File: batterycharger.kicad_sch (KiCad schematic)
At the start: 0 parts

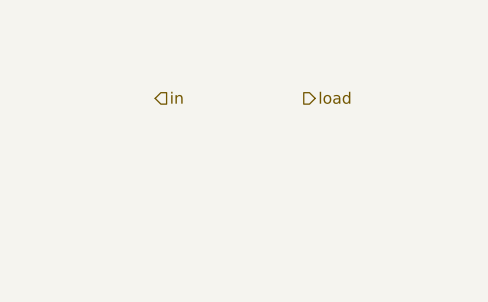
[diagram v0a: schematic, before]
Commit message: added
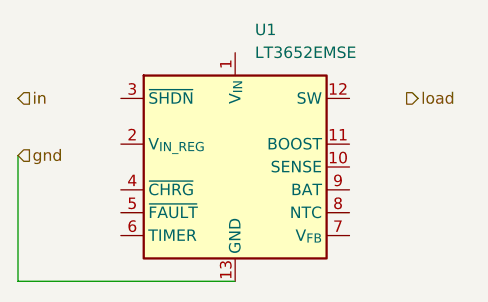
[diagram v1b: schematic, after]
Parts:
- added U1: LT3652EMSE, Package_SO:MSOP-12-1EP_3x4mm_P0.65mm_EP1.65x2.85mm, symbol Battery_Management:LT3652EMSE
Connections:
- new net gnd: U1.13 (GND)
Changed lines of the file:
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@@
 (kicad_sch (version 20230121) (generator eeschema)
   (paper "A4")
-  (hierarchical_label "in" (shape input) (at 78.74 87.63 0) (fields_autoplaced)
+  (wire (pts (xy 63.5 107.95) (xy 87.63 107.95))
+    (stroke (width 0) (type default))
+  )
+  (wire (pts (xy 63.5 93.98) (xy 63.5 107.95))
+    (stroke (width 0) (type default))
+  )
+  (hierarchical_label "in" (shape input) (at 63.5 87.63 0) (fields_autoplaced)
     (effects (font (size 1.27 1.27)) (justify left))
   )
-  (hierarchical_label "load" (shape output) (at 95.25 87.63 0) (fields_autoplaced)
+  (hierarchical_label "gnd" (shape input) (at 63.5 93.98 0) (fields_autoplaced)
     (effects (font (size 1.27 1.27)) (justify left))
   )
+  (hierarchical_label "load" (shape output) (at 106.68 87.63 0) (fields_autoplaced)
+    (effects (font (size 1.27 1.27)) (justify left))
+  )
+  (symbol (lib_id "Battery_Management:LT3652EMSE") (at 87.63 95.25 0) (unit 1)
+    (in_bom yes) (on_board yes) (dnp no) (fields_autoplaced)
+    (property "Reference" "U1" (at 89.8241 80.01 0)
+      (effects (font (size 1.27 1.27)) (justify left))
+    )
+    (property "Value" "LT3652EMSE" (at 89.8241 82.55 0)
+      (effects (font (size 1.27 1.27)) (justify left))
+    )
+    (property "Footprint" "Package_SO:MSOP-12-1EP_3x4mm_P0.65mm_EP1.65x2.85mm" (at 87.63 110.49 0)
+      (effects (font (size 1.27 1.27)) hide)
+    )
+    (property "Datasheet" "https://www.analog.com/media/en/technical-documentation/data-sheets/3652fe.pdf" (at 102.87 115.57 0)
+      (effects (font (size 1.27 1.27)) hide)
+    )
+    (pin "1")
+    (pin "10")
+    (pin "11")
+    (pin "12")
+    (pin "13")
+    (pin "2")
+    (pin "3")
+    (pin "4")
+    (pin "5")
+    (pin "6")
+    (pin "7")
+    (pin "8")
+    (pin "9")
+    (instances
+      (project "eps"
+        (path "/d1becec8-2a81-45a7-bfc6-f9ad93456edc/a41c2f06-c716-4d4c-abbd-50372b3cec58"
+          (reference "U1") (unit 1)
+        )
+        (path "/d1becec8-2a81-45a7-bfc6-f9ad93456edc/98043307-5f00-404c-bb35-46ff24bbd3b8"
+          (reference "U2") (unit 1)
+        )
+      )
+    )
+  )
 )

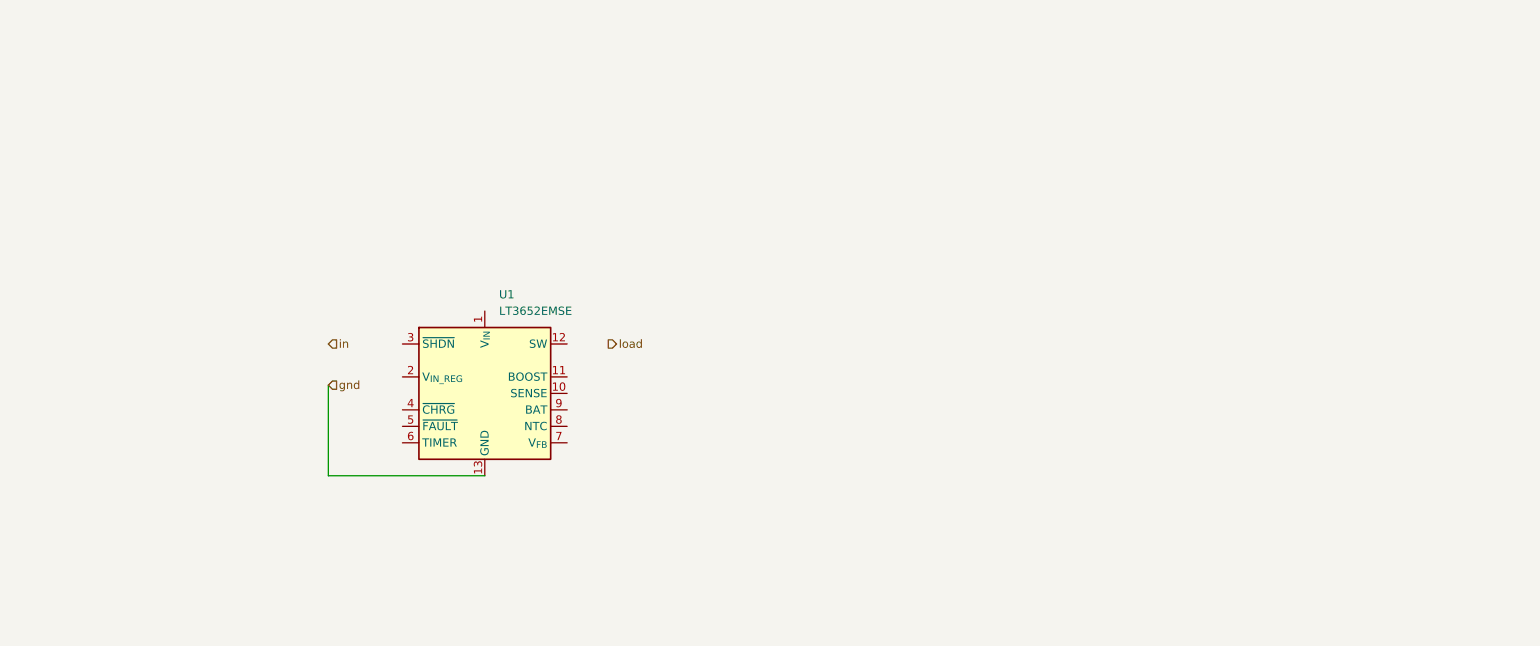
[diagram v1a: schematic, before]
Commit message: v0.1Hydrogen
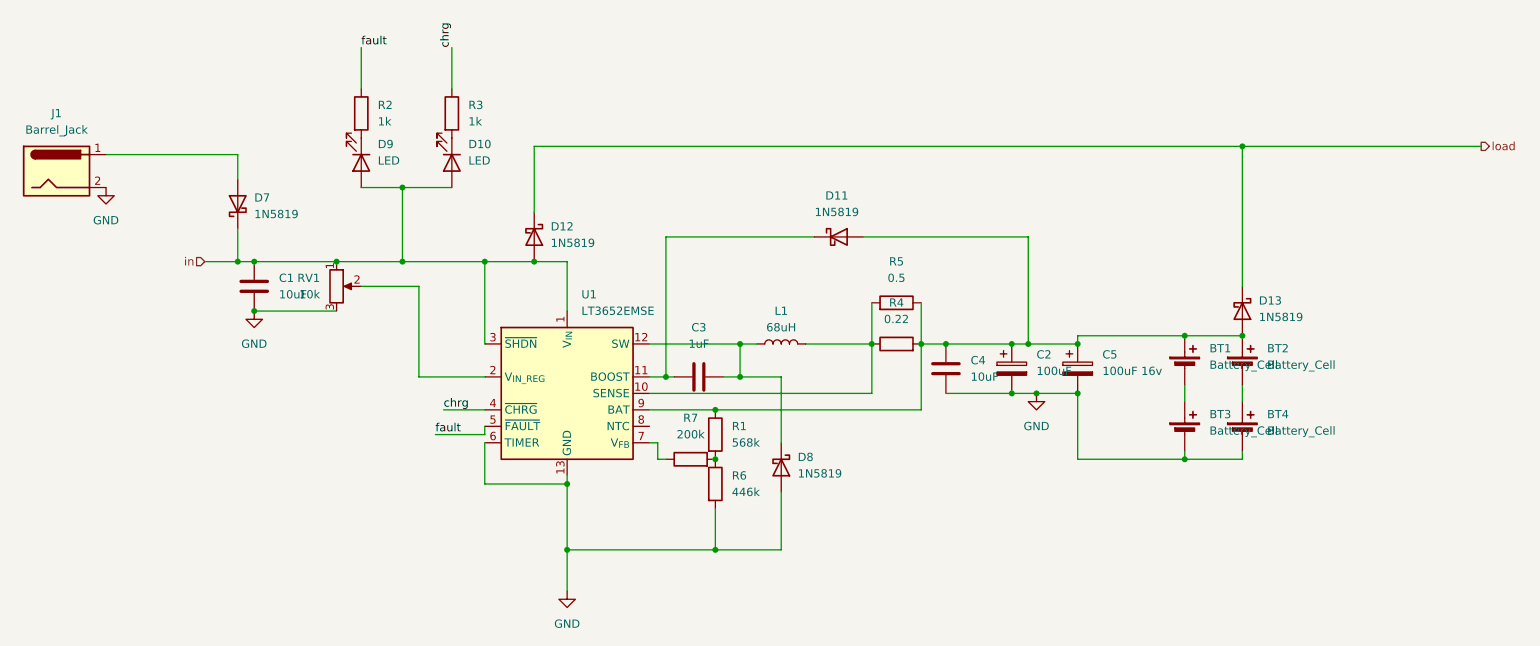
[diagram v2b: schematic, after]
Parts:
- added BT1, BT2, BT3, BT4: Battery_Cell, Battery:BatteryHolder_Keystone_1042_1x18650, symbol Device:Battery_Cell
- added C1, C4: 10uF, Capacitor_THT:C_Disc_D5.1mm_W3.2mm_P5.00mm, symbol Device:C
- added C2: 100uF, Capacitor_THT:CP_Radial_D6.3mm_P2.50mm, symbol Device:C_Polarized
- added C3: 1uF, Capacitor_THT:C_Disc_D5.0mm_W2.5mm_P2.50mm, symbol Device:C
- added C5: 100uF 16v, Capacitor_THT:CP_Radial_D6.3mm_P2.50mm, symbol Device:C_Polarized
- added D10, D9: LED, LED_THT:LED_Rectangular_W3.0mm_H2.0mm, symbol Device:LED
- added D11, D12, D13, D7, D8: 1N5819, Diode_THT:D_DO-41_SOD81_P10.16mm_Horizontal, symbol Diode:1N5819
- added J1: Barrel_Jack, Connector_BarrelJack:BarrelJack_SwitchcraftConxall_RAPC10U_Horizontal, symbol Connector:Barrel_Jack
- added L1: 68uH, Inductor_THT:L_Axial_L5.0mm_D3.6mm_P10.00mm_Horizontal_Murata_BL01RN1A2A2, symbol Device:L
- added R1: 568k, Resistor_THT:R_Axial_DIN0204_L3.6mm_D1.6mm_P5.08mm_Horizontal, symbol Device:R
- added R2, R3: 1k, Resistor_THT:R_Axial_DIN0204_L3.6mm_D1.6mm_P5.08mm_Horizontal, symbol Device:R
- added R4: 0.22, Resistor_THT:R_Axial_DIN0204_L3.6mm_D1.6mm_P5.08mm_Horizontal, symbol Device:R
- added R5: 0.5, Resistor_THT:R_Axial_DIN0204_L3.6mm_D1.6mm_P5.08mm_Horizontal, symbol Device:R
- added R6: 446k, Resistor_THT:R_Axial_DIN0204_L3.6mm_D1.6mm_P5.08mm_Horizontal, symbol Device:R
- added R7: 200k, Resistor_THT:R_Axial_DIN0204_L3.6mm_D1.6mm_P5.08mm_Horizontal, symbol Device:R
- added RV1: 10k, Potentiometer_THT:Potentiometer_Bourns_3386P_Vertical, symbol Device:R_Potentiometer
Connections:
- net gnd is gone; now on net GND: U1.13 (GND)
- net in: now also U1.1 (V_{IN}), U1.3 (~{SHDN}), C1.1, D10.2 (A), D12.2 (A), D7.1 (K), D9.2 (A), RV1.1
- net load: now also D12.1 (K), D13.1 (K)
- net at U1.10 (SENSE): now also L1.2, R4.1, R5.2
- net at U1.11 (BOOST): now also C3.1, D11.1 (K)
- net at U1.12 (SW): now also C3.2, D8.1 (K), L1.1
- net at U1.2 (V_{IN_REG}): now also RV1.2
- net chrg: now reaches U1.4 (~{CHRG})
- net chrg: now also R3.1
- net fault: now reaches U1.5 (~{FAULT})
- net fault: now also R2.1
- net GND: now reaches U1.6 (TIMER)
- net GND: now also BT3.2 (-), BT4.2 (-), C1.2, C2.2, C4.2, C5.2, D8.2 (A), J1.2, R6.2, RV1.3
- net at U1.7 (V_{FB}): now also R7.1
- net at U1.9 (BAT): now also BT1.1 (+), BT2.1 (+), C2.1, C4.1, C5.1, D11.2 (A), D13.2 (A), R1.1, R4.2, R5.1
- new net: D7.2 (A), J1.1
- new net: R1.2, R6.1, R7.2
- new net: D10.1 (K), R3.2
- new net: D9.1 (K), R2.2
- new net: BT2.2 (-), BT4.1 (+)
- new net: BT1.2 (-), BT3.1 (+)
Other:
- moved on the sheet: U1
